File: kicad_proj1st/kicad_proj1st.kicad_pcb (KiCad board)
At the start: 4 copper layers, 58 x 52.5 mm, 41 parts, among them J1 Conn_01x02, J2 Conn_01x05, J3 Conn_01x02, J4 Conn_01x02, J5 Conn_01x02, J6 Conn_01x02, J7 Conn_01x06, Q1 TSM2302CX, Q2 TSM2302CX, Q3 TSM2302CX, Q4 TSM2302CX, U1 MPU-6050, U2 VL53L0CXV0DH1, U3 TPS61089

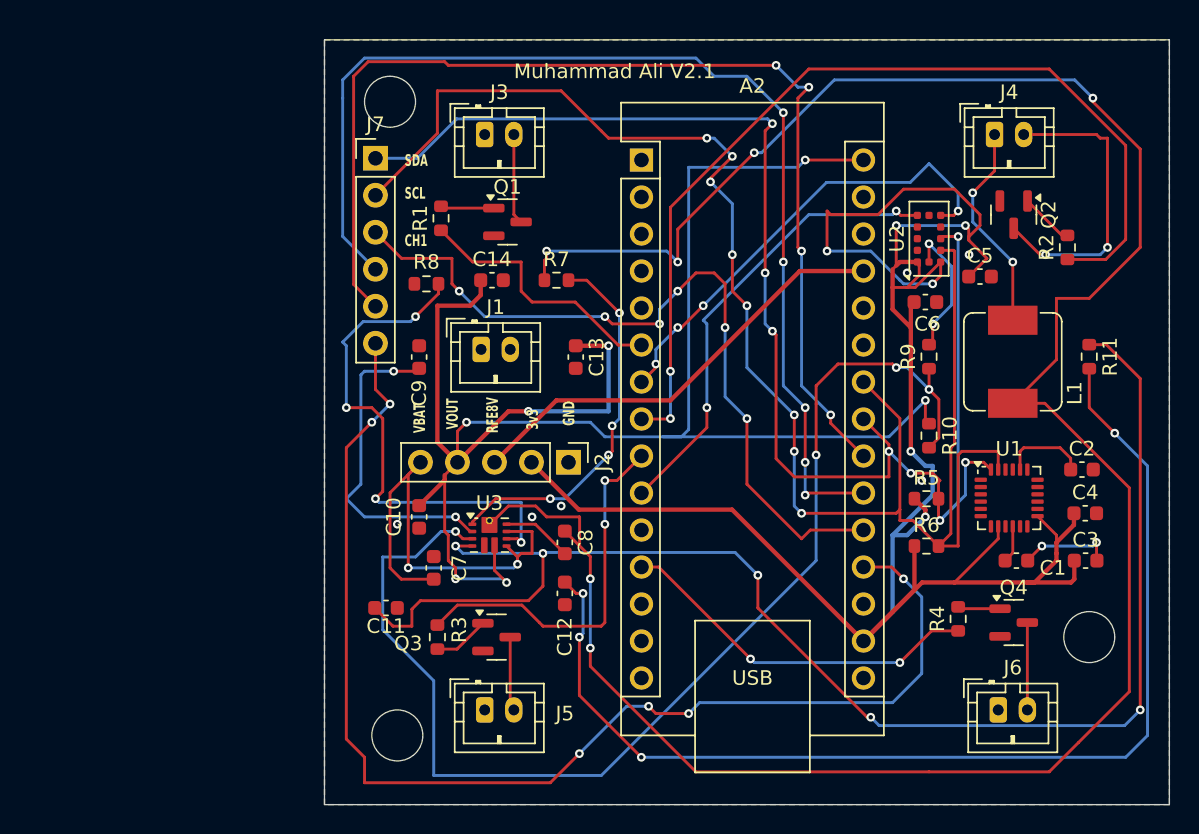
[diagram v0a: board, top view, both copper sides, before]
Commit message: Prototype 2 fin?
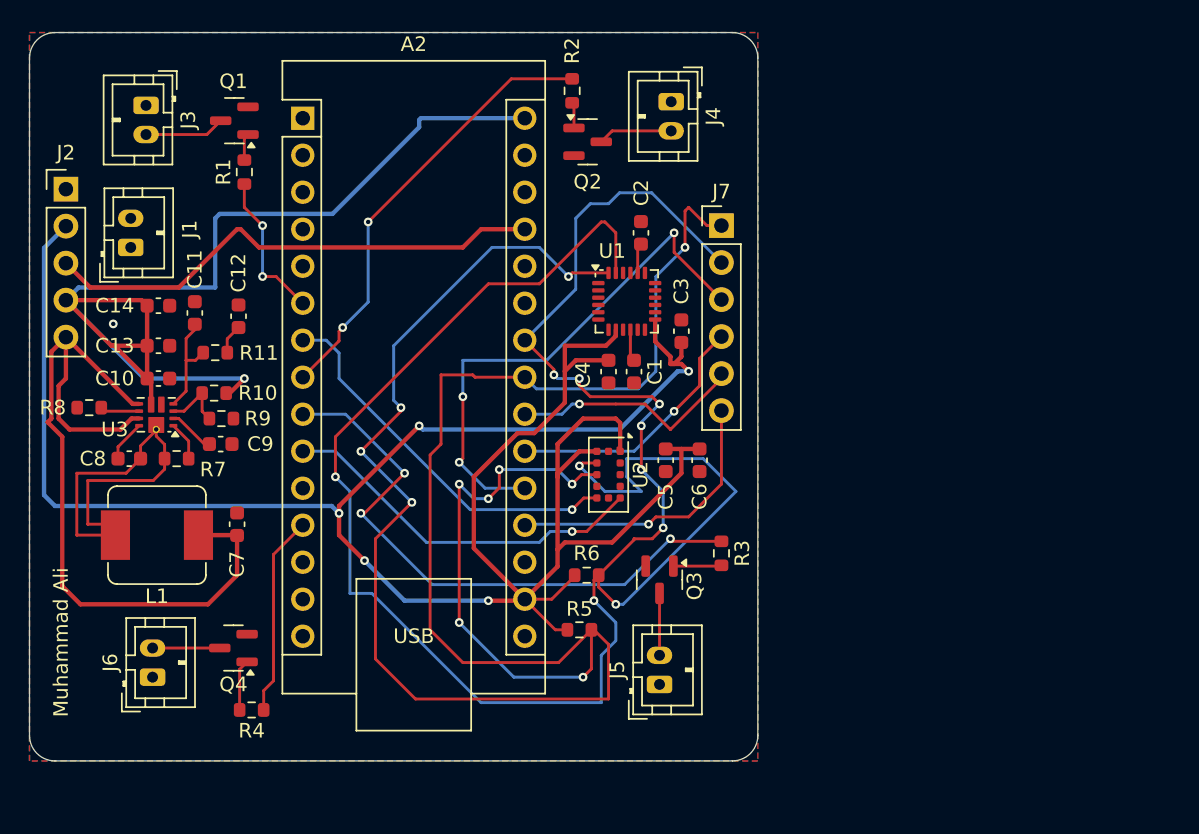
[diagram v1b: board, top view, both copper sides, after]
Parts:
- C5: value .1uC -> .1uF
- C6: value 4.7uC -> 4.7uF
- moved R11 60.0 mm to (70.2, 71.0), turned to 0 degrees
- moved L1 59.9 mm to (66.2, 83.5), turned to 180 degrees
- moved J6 58.1 mm to (66.0, 93.2), turned to 90 degrees
- moved Q4 53.6 mm to (71.5, 91.2), turned to 180 degrees
- moved R10 49.2 mm to (70.2, 73.8), turned to 180 degrees
- moved R4 48.9 mm to (72.8, 95.5), turned to 180 degrees
- moved R9 48.8 mm to (70.7, 75.5), turned to 0 degrees
- moved J2 39.3 mm to (60.0, 59.8), turned to 0 degrees
- moved R2 35.7 mm to (94.8, 53.0), turned to -90 degrees
- moved C2 34.4 mm to (99.5, 62.8), turned to 90 degrees
- moved C4 34.1 mm to (97.2, 72.3), turned to -90 degrees
- moved C3 31.9 mm to (102.2, 69.5), turned to 90 degrees
- moved C8 30.4 mm to (64.3, 78.2), turned to 180 degrees
- moved Q2 29.7 mm to (95.8, 56.5), turned to 0 degrees
- moved U1 29.5 mm to (98.5, 67.5)
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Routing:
- net Net-(U3-SW): track 159.8 -> 28.5 mm, vias 6 -> 0
- net Net-(U3-COMP): track 98.4 -> 7.47 mm, vias 5 -> 0
- net Net-(U3-FB): track 83.0 -> 4.45 mm, vias 4 -> 0
- net Net-(C12-Pad1): track 76.9 -> 2.05 mm, vias 4 -> 0
- net CH4: track 84.2 -> 19.7 mm, vias 6 -> 1
- net SDA: track 100.1 -> 162.8 mm, vias 8 -> 11
- net CH3: track 76.3 -> 16.3 mm, vias 4 -> 1
- net CH2: track 77.8 -> 17.9 mm, vias 5 -> 1
- net V_OUT: track 122.6 -> 78.8 mm, vias 7 -> 1
- net SCL: track 112.9 -> 150.7 mm, vias 8 -> 10
- net /Motor Switch2: track 64.9 -> 30.6 mm
- net Net-(U3-ILIM): track 35.7 -> 2.70 mm, vias 4 -> 0
- net Net-(U3-FSW): track 25.9 -> 2.69 mm, vias 4 -> 0
- net Net-(U3-VCC): track 22.7 -> 3.20 mm, vias 2 -> 0
- net CH1: track 54.1 -> 36.4 mm, vias 6 -> 3
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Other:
- board size 58 x 52.5 mm -> 50 x 50 mm
- board text added: "Muhammad Ali"
- board text removed: "3v3"
- board text removed: "CH1"
- board text removed: "GND"
- board text removed: "Muhammad Ali V2.1"
- board text removed: "RFE8V"
- board text removed: "SCL"
- board text removed: "SDA"
- board text removed: "VBAT"
- board text removed: "VOUT"
